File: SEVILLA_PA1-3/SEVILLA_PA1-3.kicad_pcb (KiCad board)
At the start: 2 copper layers, 64 x 46 mm, 10 parts, among them SW3 SW_SPST, SW4 SW_SPST, U1 HDSP-7401, U2 PIC16F84A-XXP, U3 HDSP-7401, Y1 4 MHz

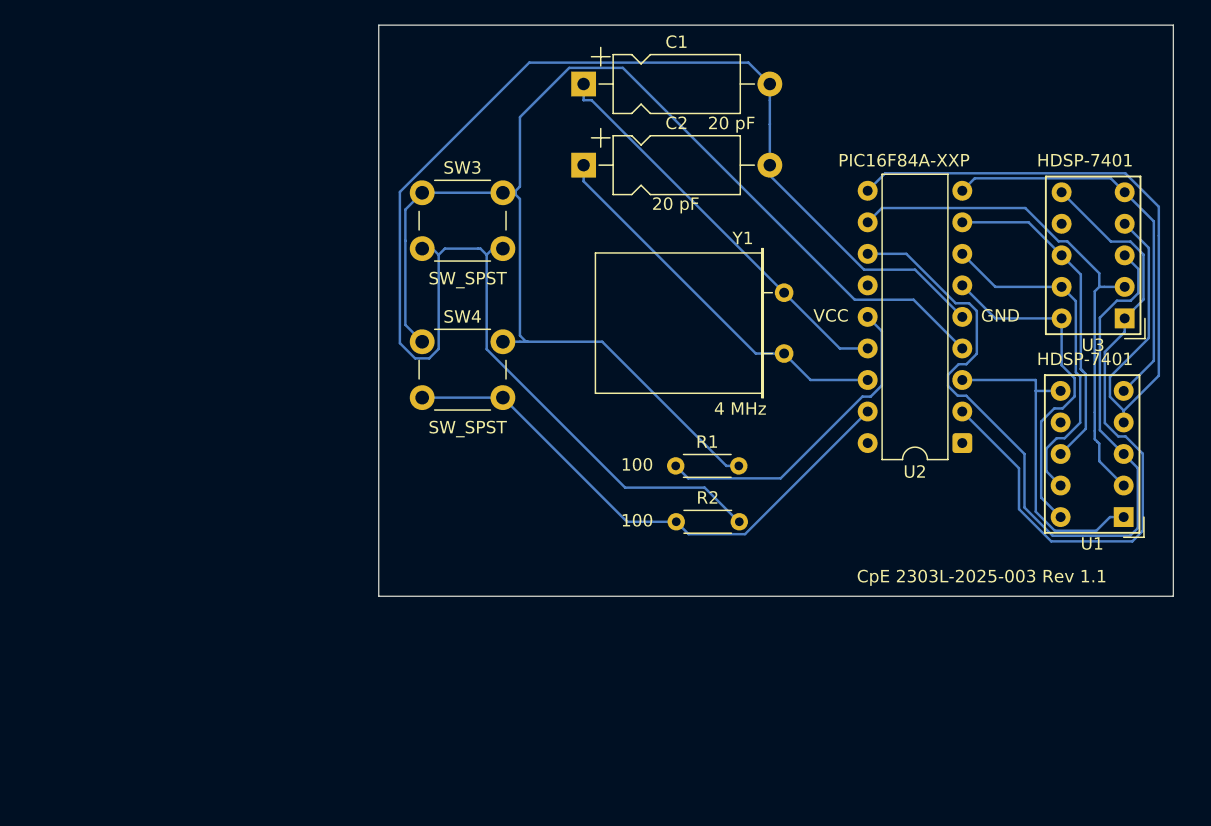
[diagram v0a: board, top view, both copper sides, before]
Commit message: Refactor code structure and remove redundant sections for improved readability and maintainability
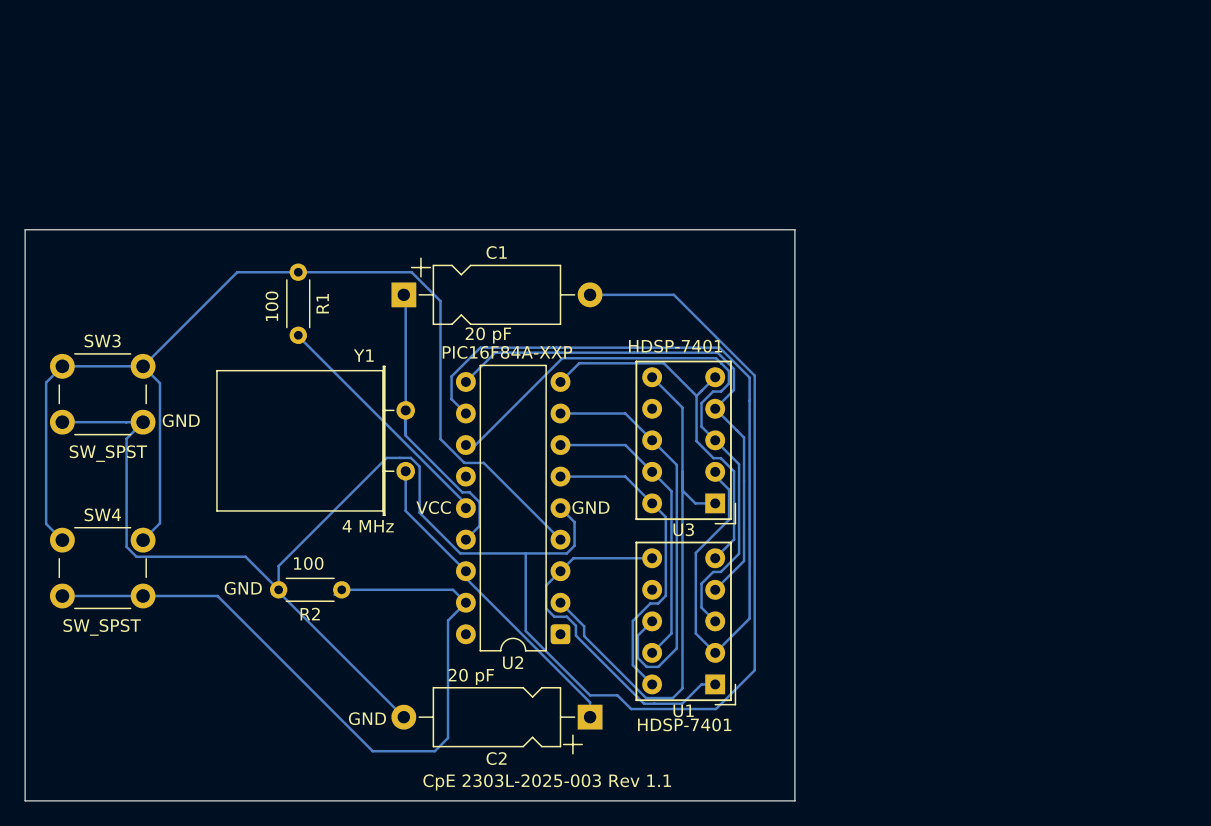
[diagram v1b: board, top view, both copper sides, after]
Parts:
- moved C2 44.5 mm to (161.0, 108.2), turned to 180 degrees
- moved U3 36.2 mm to (171.1, 91.0)
- moved U2 35.8 mm to (158.6, 101.6)
- moved U1 35.6 mm to (171.1, 105.6)
- moved SW4 33.1 mm to (118.5, 94.0)
- moved SW3 32.2 mm to (118.5, 80.0)
- moved R1 32.2 mm to (137.5, 77.5), turned to 90 degrees
- moved Y1 31.9 mm to (146.2, 83.5)
- moved R2 27.5 mm to (141.0, 98.0), turned to 180 degrees
- moved C1 22.3 mm to (146.0, 74.2)
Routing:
- net Net-(U1-F): track 41.6 -> 69.5 mm
- net GND: track 127.1 -> 152.1 mm
- net Net-(SW3-A): track 109.1 -> 88.9 mm
- net Net-(U1-E): track 61.3 -> 43.4 mm
- net Net-(U1-G): track 66.8 -> 49.3 mm
- net Net-(SW4-B): track 44.5 -> 59.4 mm
- net Net-(U2-RA3): track 55.0 -> 44.4 mm
- net Net-(U2-OSC2/CLKOUT): track 32.5 -> 24.9 mm
- net VCC: track 26.1 -> 19.5 mm
- net Net-(U1-C): track 27.0 -> 33.3 mm
- net Net-(U2-OSC1/CLKIN): track 30.8 -> 26.0 mm
- net Net-(U1-B): track 27.7 -> 24.1 mm
- net Net-(U2-TOCKI/RA4): track 26.7 -> 29.2 mm
- net Net-(U1-A): track 27.7 -> 25.4 mm
- net Net-(U1-D): track 31.9 -> 30.1 mm
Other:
- board size 64 x 46 mm -> 62 x 46 mm
